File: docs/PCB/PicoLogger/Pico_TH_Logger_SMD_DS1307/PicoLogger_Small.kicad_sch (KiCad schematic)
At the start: 24 parts, among them J1 Sensor, J2 LCD 16x2, J3 Additional connector, J5 SPI, SW1 SW_Push, SW2 SW_Push, U1 DS1307Z+, Y1 Crystal

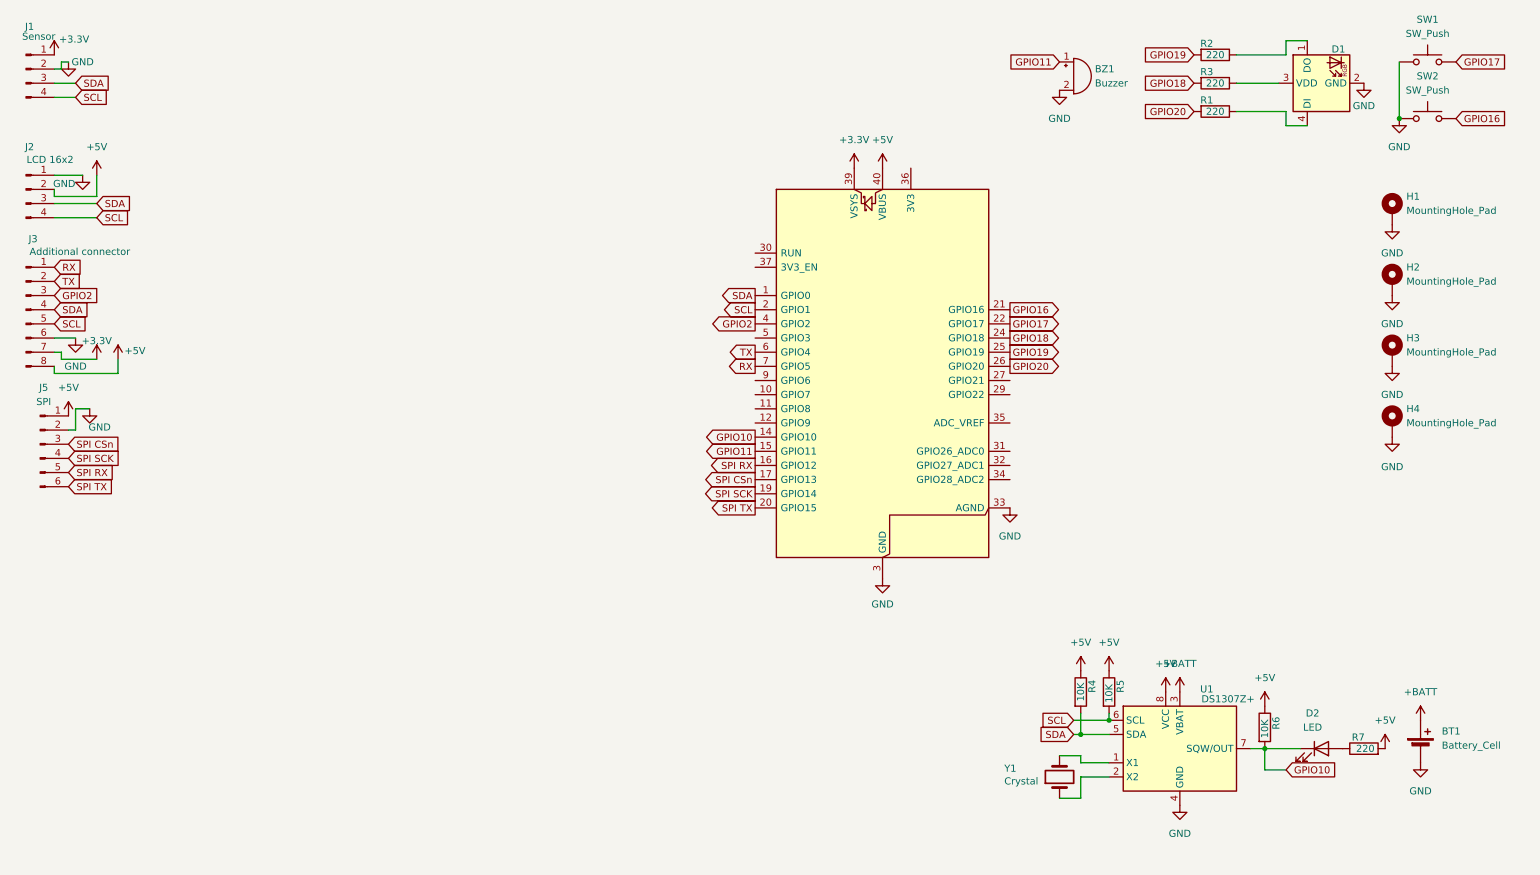
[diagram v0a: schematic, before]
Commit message: Updated docs.
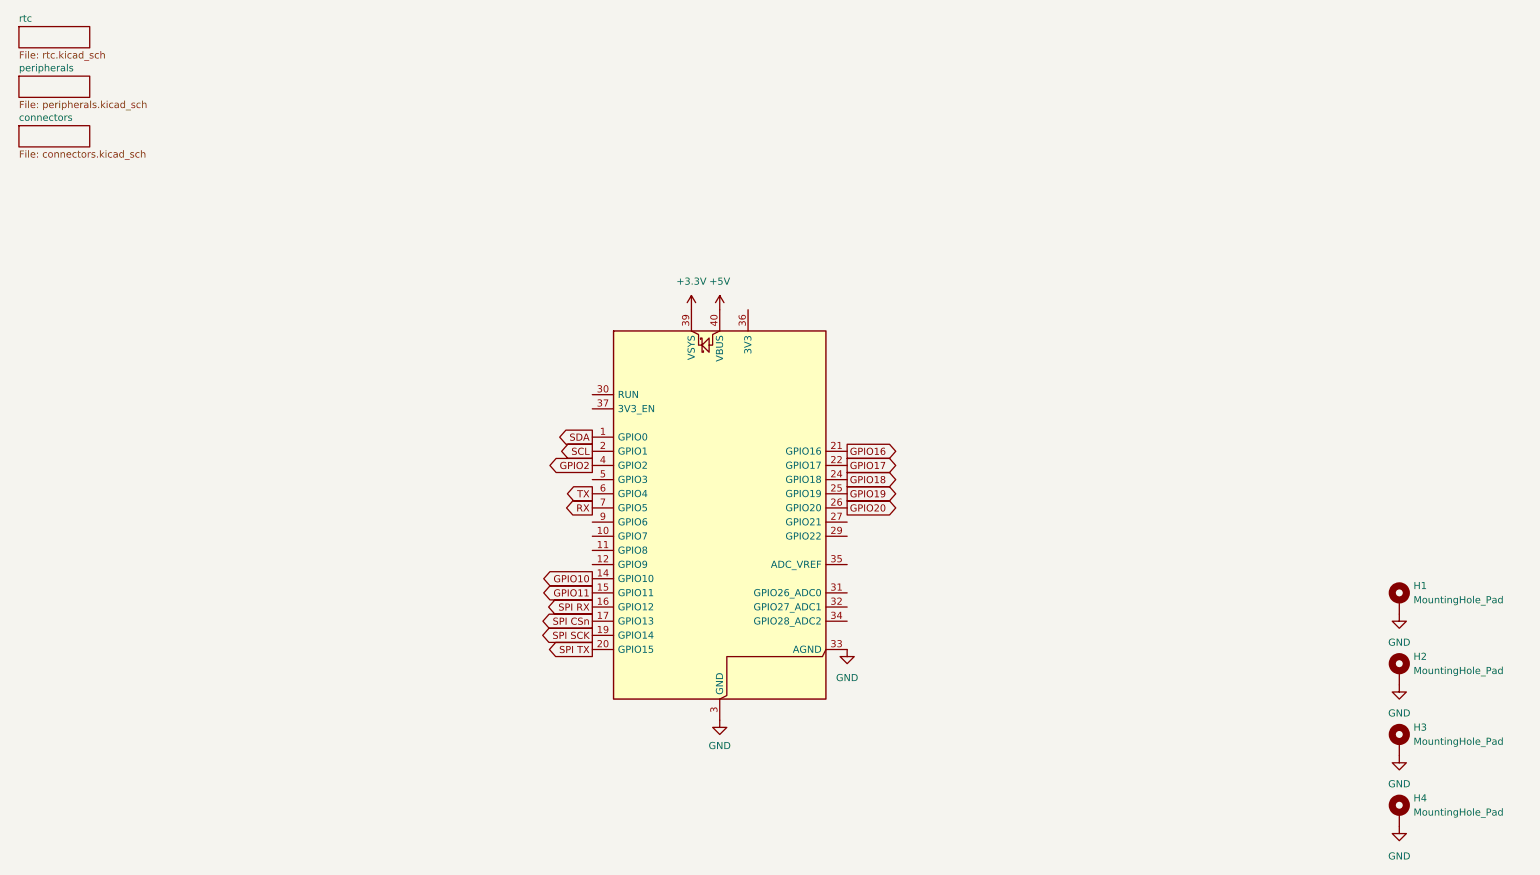
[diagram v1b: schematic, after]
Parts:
- removed BT1: Battery_Cell, Battery:BatteryHolder_Keystone_104_1x23mm, symbol Device:Battery_Cell
- removed BZ1: Buzzer, Buzzer_Beeper:Buzzer_12x9.5RM7.6, symbol Device:Buzzer
- removed D1: APA-106-F5, LED_SMD:LED_Avago_PLCC4_3.2x2.8mm_CW, symbol LED:APA-106-F5
- removed D2: LED, LED_SMD:LED_0805_2012Metric, symbol Device:LED
- removed J1: Sensor, Connector_PinHeader_2.54mm:PinHeader_1x04_P2.54mm_Vertical, symbol Connector:Conn_01x04_Pin
- removed J2: LCD 16x2, Connector_PinHeader_2.54mm:PinHeader_1x04_P2.54mm_Vertical, symbol Connector:Conn_01x04_Pin
- removed J3: Additional connector, Connector_PinHeader_2.54mm:PinHeader_1x08_P2.54mm_Horizontal, symbol Connector:Conn_01x08_Pin
- removed J5: SPI, Connector_PinHeader_2.54mm:PinHeader_1x06_P2.54mm_Horizontal, symbol Connector:Conn_01x06_Pin
- removed R1, R2, R3, R7: 220, Resistor_SMD:R_0805_2012Metric, symbol Device:R
- removed R4, R5, R6: 10K, Resistor_SMD:R_0805_2012Metric, symbol Device:R
- removed SW1, SW2: SW_Push, Button_Switch_THT:SW_PUSH_6mm, symbol Switch:SW_Push
- removed U1: DS1307Z+, Package_SO:SOIC-8_3.9x4.9mm_P1.27mm, symbol Timer_RTC:DS1307Z+
- removed Y1: Crystal, Crystal:Crystal_SMD_3215-2Pin_3.2x1.5mm, symbol Device:Crystal
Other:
- added sheet connectors (connectors.kicad_sch)
- added sheet peripherals (peripherals.kicad_sch)
- added sheet rtc (rtc.kicad_sch)
- company: (none) -> Creator: Piotr Kłyś
- title: (none) -> Raspberry Pi Pico Logger
- moved on the sheet: H1, H2, H3, H4
